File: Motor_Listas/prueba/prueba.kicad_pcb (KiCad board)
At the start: 2 copper layers, 1 part

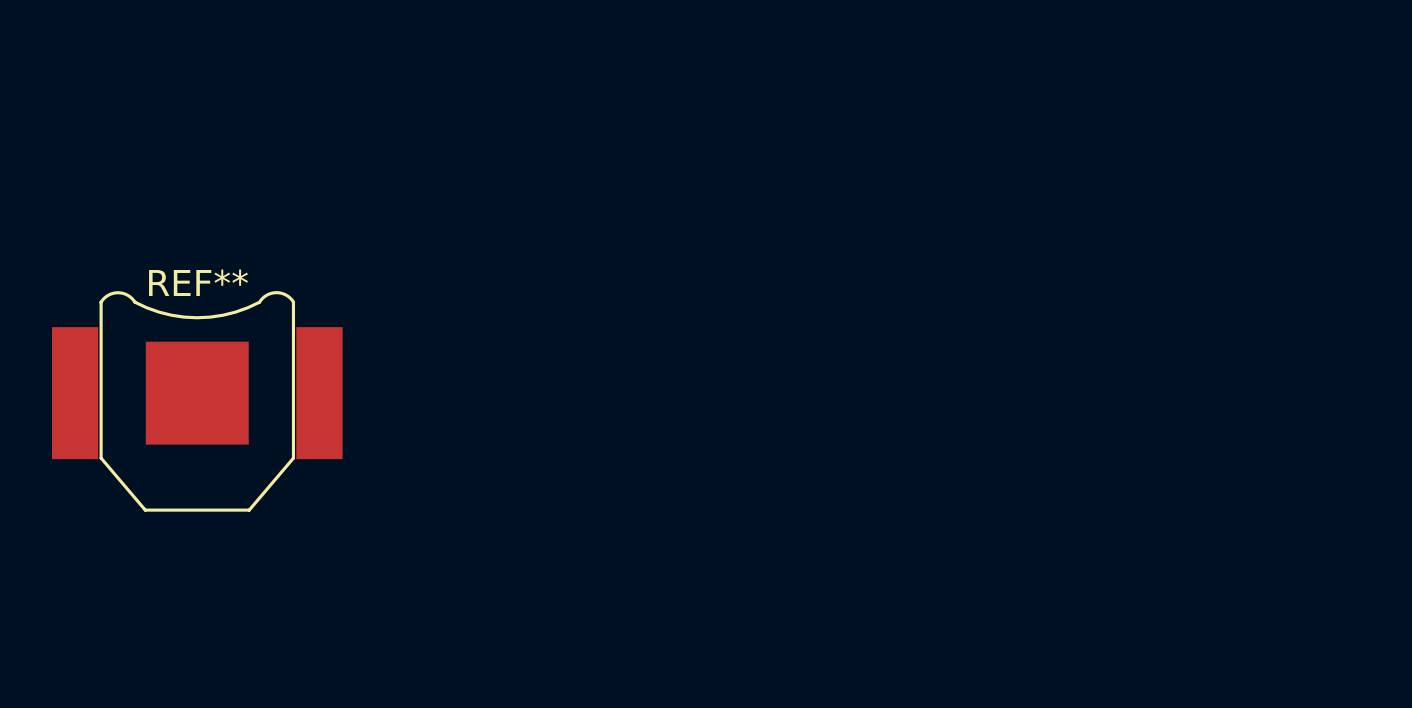
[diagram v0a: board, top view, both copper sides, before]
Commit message: first attemp
it start to work
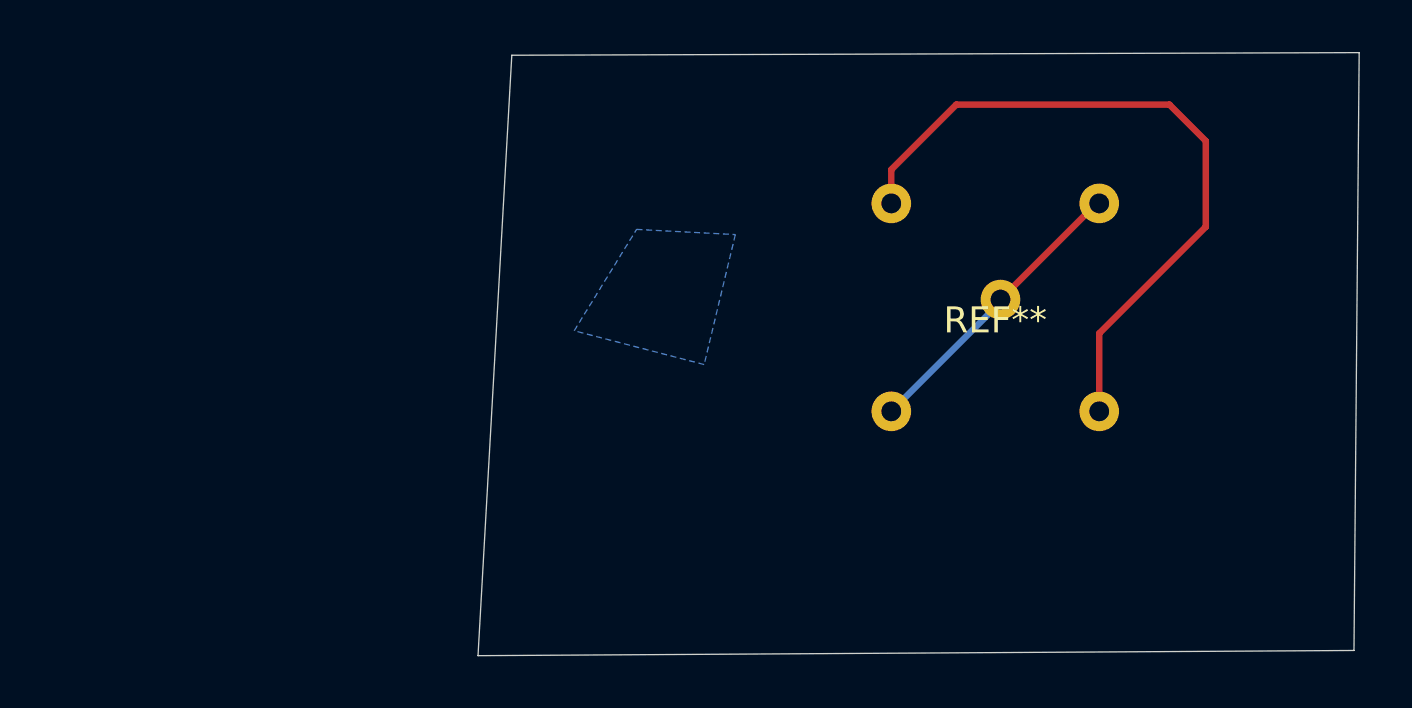
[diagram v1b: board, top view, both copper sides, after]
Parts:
- removed the REF** at (82.8, 28.8)
- added REF**: prueba, prueba:prueba, F.Cu at (113.5, 25.5)
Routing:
- net (no net): track 0.00 -> 38.5 mm
- added copper zone on B.Cu, net (none)
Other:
- board outline added: 33.9 x 23.2 mm
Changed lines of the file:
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@@
   (general
     (thickness 1.6)
-    (drawings 0)
-    (tracks 0)
+    (drawings 4)
+    (tracks 11)
     (zones 0)
     (modules 1)
@@
     (uvia_drill 0.1)
   )
-  (module Battery:BatteryHolder_Keystone_2998_1x6.8mm (layer F.Cu)
-    (at 82.8 28.8)
-    (descr www.keyelco.com/product-pdf.cfm?p=763)
-    (tags "Keystone type 2998 battery holder")
-    (attr smd)
-    (fp_text reference REF** (at 0 -4.2) (layer F.SilkS)
+  (module prueba:prueba (layer F.Cu)
+    (at 113.5 25.5)
+    (fp_text reference REF** (at 0 0.5) (layer F.SilkS)
       (effects (font (size 1 1) (thickness 0.15)))
     )
-    (fp_text value BatteryHolder_Keystone_2998_1x6.8mm (at 0 5.725) (layer F.Fab)
+    (fp_text value prueba (at 0 -0.5) (layer F.Fab)
       (effects (font (size 1 1) (thickness 0.15)))
     )
-    (fp_arc (start 3.05 -3.15) (end 3.6 -3.44) (angle -125.2183105) (layer F.Fab) (width 0.1))
-    (fp_arc (start 0 -8.03) (end -2.5 -3.43) (angle -56.6) (layer F.Fab) (width 0.1))
-    (fp_text user %R (at 0.1 4) (layer F.Fab)
-      (effects (font (size 0.7 0.7) (thickness 0.15)))
-    )
-    (fp_arc (start 0 -8) (end -2.4 -3.5) (angle -56.03531623) (layer F.SilkS) (width 0.12))
-    (fp_arc (start 3.05 -3.1) (end 3.703723 -3.5) (angle -117.603575) (layer F.SilkS) (width 0.12))
-    (fp_arc (start -3.05 -3.1) (end -2.4 -3.5) (angle -117.603575) (layer F.SilkS) (width 0.12))
-    (fp_arc (start -3.05 -3.17) (end -2.5 -3.42) (angle -133) (layer F.Fab) (width 0.12))
-    (fp_circle (center 0 0) (end 3.4 0) (layer Dwgs.User) (width 0.1))
-    (fp_line (start -3.7 -3.5) (end -3.7 2.5) (layer F.SilkS) (width 0.12))
-    (fp_line (start 3.7 -3.5) (end 3.7 2.5) (layer F.SilkS) (width 0.12))
-    (fp_line (start -2 4.5) (end 2 4.5) (layer F.SilkS) (width 0.12))
-    (fp_line (start 2 4.5) (end 3.7 2.5) (layer F.SilkS) (width 0.12))
-    (fp_line (start -2 4.5) (end -3.7 2.5) (layer F.SilkS) (width 0.12))
-    (fp_line (start -5.9 -5.1) (end -5.9 4.8) (layer F.CrtYd) (width 0.05))
-    (fp_line (start -5.9 4.8) (end 5.9 4.8) (layer F.CrtYd) (width 0.05))
-    (fp_line (start 5.9 4.8) (end 5.9 -5.1) (layer F.CrtYd) (width 0.05))
-    (fp_line (start 5.9 -5.1) (end -5.9 -5.1) (layer F.CrtYd) (width 0.05))
-    (fp_line (start -3.6 -3.4) (end -3.6 2.4) (layer F.Fab) (width 0.1))
-    (fp_line (start 3.6 2.45) (end 3.6 -3.5) (layer F.Fab) (width 0.1))
-    (fp_line (start 1.95 4.4) (end 3.6 2.45) (layer F.Fab) (width 0.1))
-    (fp_line (start -1.95 4.4) (end 1.95 4.4) (layer F.Fab) (width 0.1))
-    (fp_line (start -3.6 2.45) (end -1.95 4.4) (layer F.Fab) (width 0.1))
-    (pad 2 smd rect (at 0 0) (size 3.96 3.96) (layers F.Cu F.Paste F.Mask))
-    (pad 1 smd rect (at 4.7 0) (size 1.78 5.08) (layers F.Cu F.Paste F.Mask))
-    (pad 1 smd rect (at -4.7 0) (size 1.78 5.08) (layers F.Cu F.Paste F.Mask))
-    (model ${KISYS3DMOD}/Battery.3dshapes/BatteryHolder_Keystone_2998_1x6.8mm.wrl
-      (at (xyz 0 0 0))
-      (scale (xyz 1 1 1))
-      (rotate (xyz 0 0 0))
+    (pad 5 thru_hole circle (at -4 -4) (size 1.524 1.524) (drill 0.762) (layers *.Cu *.Mask))
+    (pad 4 thru_hole circle (at -4 4) (size 1.524 1.524) (drill 0.762) (layers *.Cu *.Mask))
+    (pad 3 thru_hole circle (at 4 4) (size 1.524 1.524) (drill 0.762) (layers *.Cu *.Mask))
+    (pad 2 thru_hole circle (at 4 -4) (size 1.524 1.524) (drill 0.762) (layers *.Cu *.Mask))
+    (pad 1 thru_hole circle (at 0.2 -0.3) (size 1.524 1.524) (drill 0.762) (layers *.Cu *.Mask))
+  )
+  (gr_line (start 93.6 38.9) (end 94.9 15.8) (layer Edge.Cuts) (width 0.05))
+  (gr_line (start 127.3 38.7) (end 93.6 38.9) (layer Edge.Cuts) (width 0.05))
+  (gr_line (start 127.5 15.7) (end 127.3 38.7) (layer Edge.Cuts) (width 0.05))
+  (gr_line (start 94.9 15.8) (end 127.5 15.7) (layer Edge.Cuts) (width 0.05))
+  (segment (start 117.4 21.5) (end 113.7 25.2) (width 0.25) (layer F.Cu) (net 0))
+  (segment (start 117.5 21.5) (end 117.4 21.5) (width 0.25) (layer F.Cu) (net 0))
+  (segment (start 117.5 29.5) (end 117.5 26.5) (width 0.25) (layer F.Cu) (net 0))
+  (segment (start 117.5 26.5) (end 121.6 22.4) (width 0.25) (layer F.Cu) (net 0))
+  (segment (start 121.6 22.4) (end 121.6 19.1) (width 0.25) (layer F.Cu) (net 0))
+  (segment (start 121.6 19.1) (end 120.2 17.7) (width 0.25) (layer F.Cu) (net 0))
+  (segment (start 120.2 17.7) (end 112 17.7) (width 0.25) (layer F.Cu) (net 0))
+  (segment (start 109.5 20.2) (end 109.5 21.5) (width 0.25) (layer F.Cu) (net 0))
+  (segment (start 112 17.7) (end 109.5 20.2) (width 0.25) (layer F.Cu) (net 0))
+  (segment (start 113.7 25.3) (end 109.5 29.5) (width 0.25) (layer B.Cu) (net 0))
+  (segment (start 113.7 25.2) (end 113.7 25.3) (width 0.25) (layer B.Cu) (net 0))
+  (zone (net 0) (net_name "") (layer B.Cu) (hatch edge 0.508)
+    (connect_pads (clearance 0.508))
+    (min_thickness 0.254)
+    (fill yes (arc_segments 32) (thermal_gap 0.508) (thermal_bridge_width 0.508))
+    (polygon
+      (pts
+        (xy 103.5 22.7) (xy 102.3 27.7) (xy 97.3 26.4) (xy 99.7 22.5)
+      )
     )
   )
